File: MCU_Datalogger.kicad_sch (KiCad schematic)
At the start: 25 parts, among them U1 24LC1025, U2 DS1337S_, U3 24LC1025, U4 ATMEGA328P-AU, Y1 32.768 KHz, Y2 16 MHz

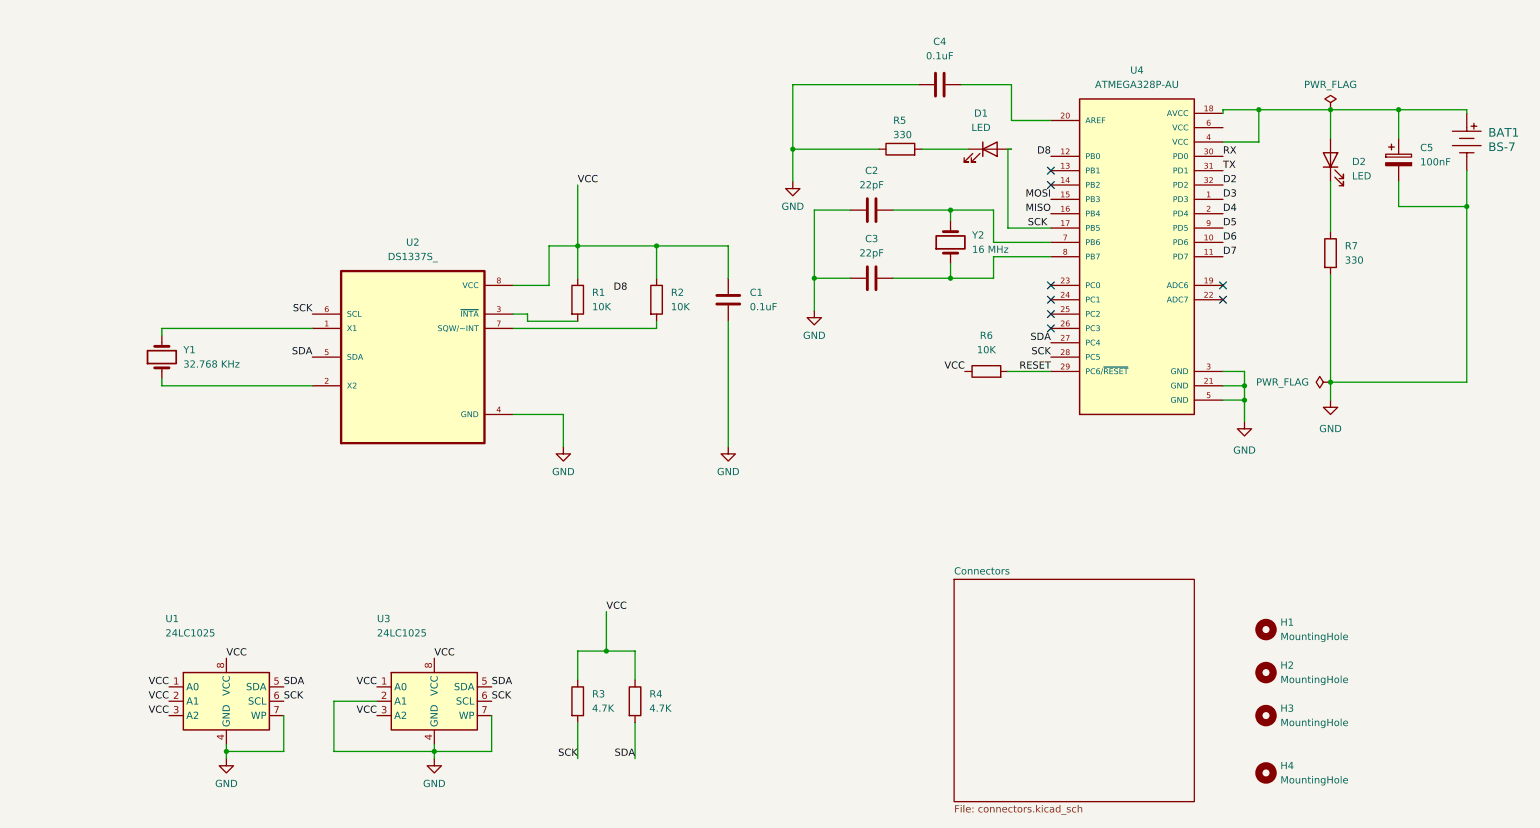
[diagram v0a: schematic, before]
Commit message: Completed comments.
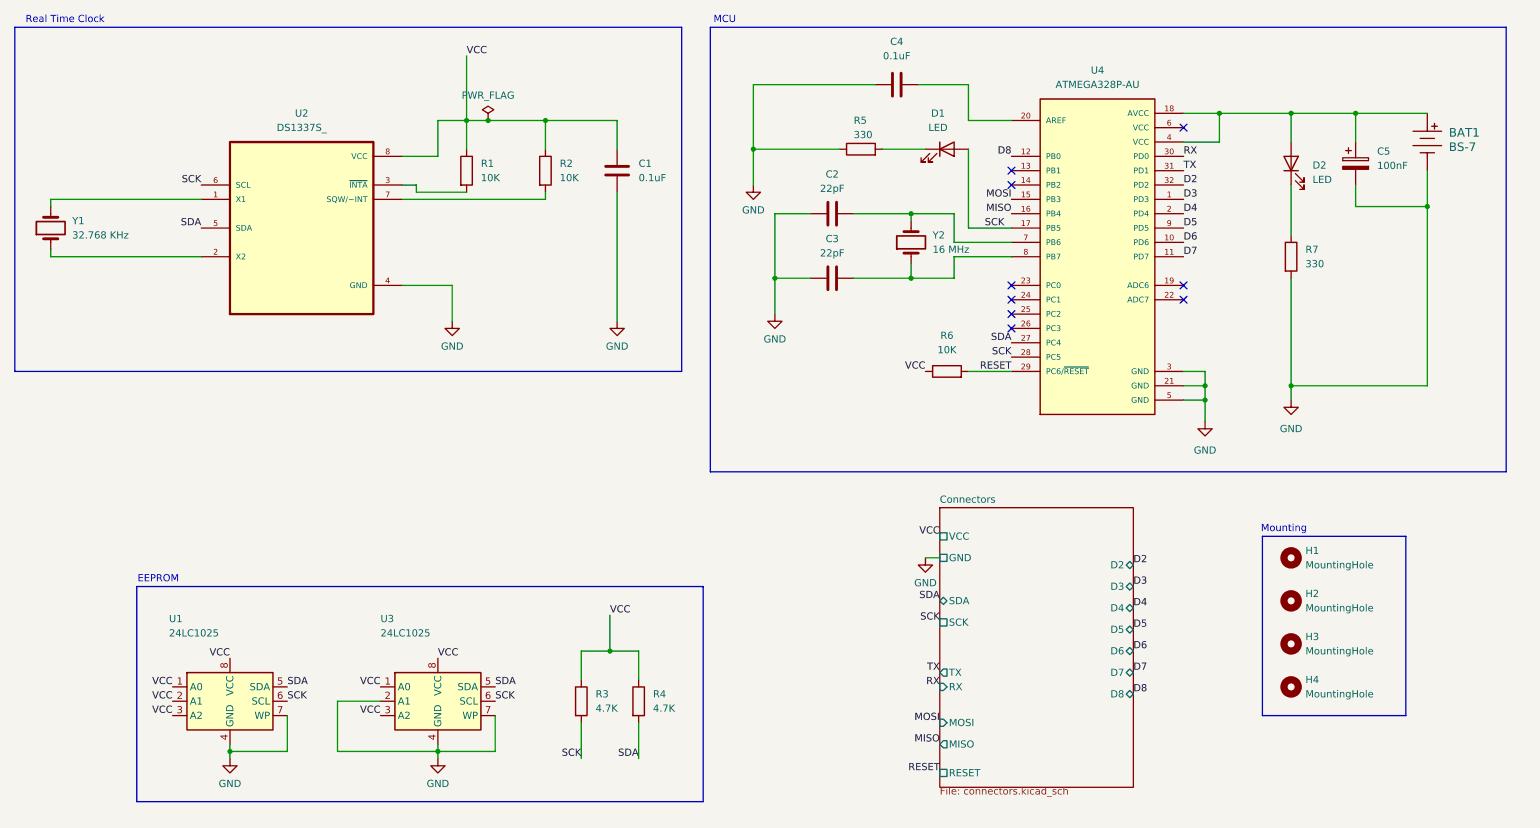
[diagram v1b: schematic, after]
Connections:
- no-connect marks 8 -> 9
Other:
- sheet Connectors ports: added D2, D3, D4, D5, D6, D7, D8, GND, MISO, MOSI, RESET, RX, SCK, SDA, TX, VCC; removed none
- note added: "EEPROM"
- note added: "MCU"
- note added: "Mounting"
- note added: "Real Time Clock"
- moved on the sheet: BAT1, C1, C2, C3, C4, C5, D1, D2, H1, H2, H3, H4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

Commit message: Completed routing.
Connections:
- net GND: now also BAT1.2; no longer BAT1.Neg
- net at C5.1, D2.2 (A), U4.18 (AVCC)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: now also BAT1.1; no longer BAT1.Pos
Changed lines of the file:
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@@
 			)
 		)
-		(pin "Neg"
+		(property "Purpose" ""
+			(at 267.97 44.45 0)
+			(effects
+				(font
+					(size 1.27 1.27)
+				)
+			)
 		)
-		(pin "Pos"
+		(pin "2"
+		)
+		(pin "1"
 		)
 		(instances
